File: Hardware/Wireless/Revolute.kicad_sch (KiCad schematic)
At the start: 55 parts, among them U1 BQ27441-G1, U2 Button, U2 nrf52833_qfn40, U3 AS5600, U4 MIC5504, U5 BQ24075RGT, U7 Conn_01x14_Socket, X1 32.768 kHz, X2 32MHZ

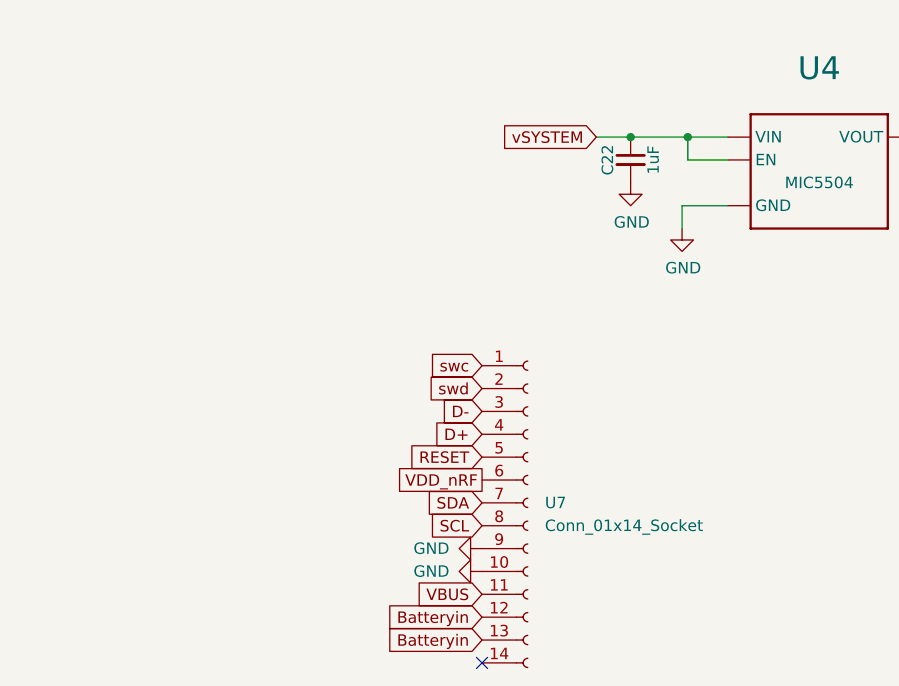
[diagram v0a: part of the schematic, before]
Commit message: current version
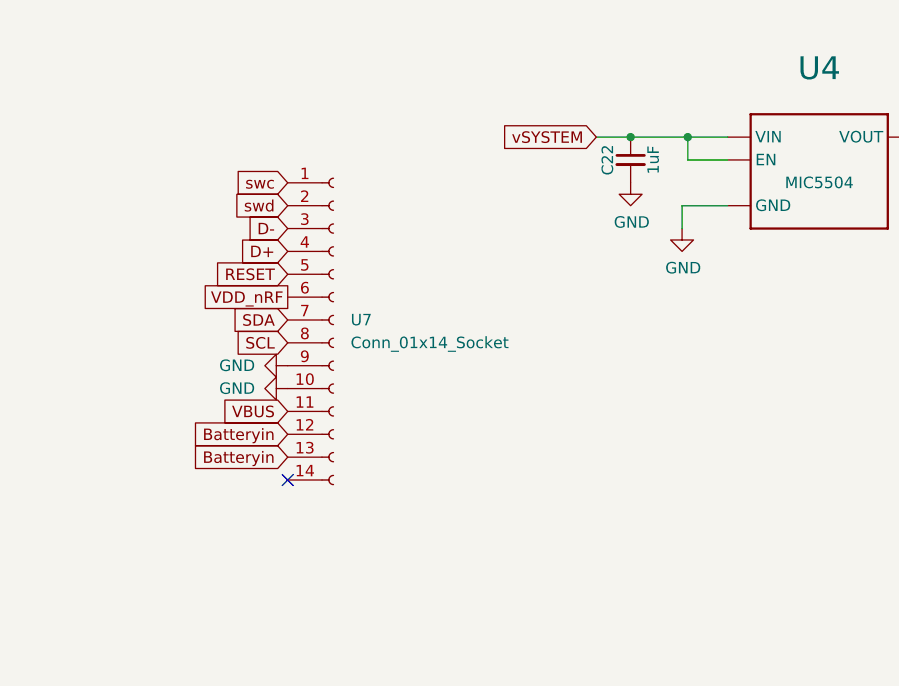
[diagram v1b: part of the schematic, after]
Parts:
- AE1: footprint RF_Antenna:Johanson_2450AT18x100 -> Library:Antenna 2450AT42A100
- C1, C6, C8: ID 16 -> 140
- C11: ID 55 -> 139
- C13, C20, C5: ID 21 -> 145
- C14: ID 26 -> 137
- C15: footprint Capacitor_SMD:C_0402_1005Metric -> Library:Capacitor-0201; ID 18 -> 146
- C16, C17, C2, C3: ID 17 -> 142
- C18: ID 56 -> 141
- C19: footprint Capacitor_SMD:C_0402_1005Metric -> Library:Capacitor-0201; ID 112 -> 144
- C21, C22, C23, C24, C4, C7, C9: ID 30 -> 136
- R1: JLC Part C25867 -> (none); LCSC Part C114759 -> (none); Manufacturer Part RC0402FR-071K5L -> (none)
- R2: footprint Library:Resistor_0402_1005M-nosilk -> Library:Resistor-0201; ID 27 -> 138; JLC Part C25867 -> (none); LCSC Part C114759 -> (none); Manufacturer Part RC0402FR-071K5L -> (none)
- R3: ID 6 -> 131; JLC Part C25867 -> (none); LCSC Part C114759 -> (none); Manufacturer Part RC0402FR-071K5L -> (none)
- R6, R8: ID 29 -> 135
- R9: ID 27 -> 138; JLC Part C25867 -> (none); LCSC Part C114759 -> (none); Manufacturer Part RC0402FR-071K5L -> (none)
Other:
- moved on the sheet: U7
